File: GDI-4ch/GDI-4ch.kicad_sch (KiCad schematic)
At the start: 311 parts, among them J1 Conn_02x02_Odd_Even, J2 FTSH-107-01-F-DV-K, J3 TC2030, J4 Conn_01x06, J5 Conn_01x06, P1 368255-2, P18 Pad, P19 Pad, P2 Pad, P20 Pad, P3 Pad, P36 Pad, P4 Pad, P5 Pad, Q1 BUK9230-100B, Q10 BUK9230-100B, Q11 BUK9230-100B, Q12 BUK9230-100B, Q13 AOD4185, Q14 VND14NV04TR-E, Q15 VND14NV04TR-E, Q16 BUK9230-100B, Q2 BUK9230-100B, Q3 BUK9230-100B, Q4 BUK9230-100B, Q5 BUK9230-100B, Q6 BUK9230-100B, Q7 BUK9230-100B, Q8 BUK9230-100B, Q9 BUK9230-100B, U1 MC33816, U2 TJA1051T-3, U3 LM78M05_TO252, U4 74HC14PW,118, U5 XC6206P332MR, U6 MCP6004, U7 GD32F103CBT6, U8 74HC14PW,118, Y1 8MHz, Y2 1MHz

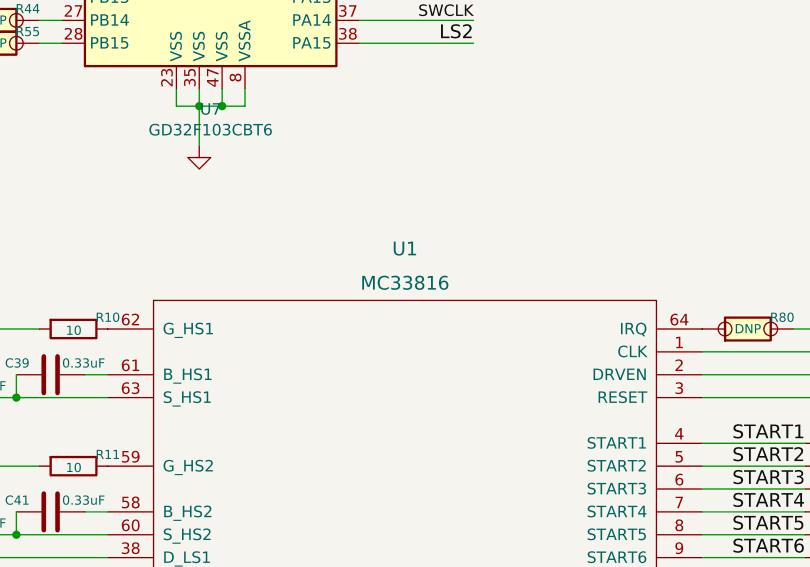
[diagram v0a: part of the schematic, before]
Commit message: #205
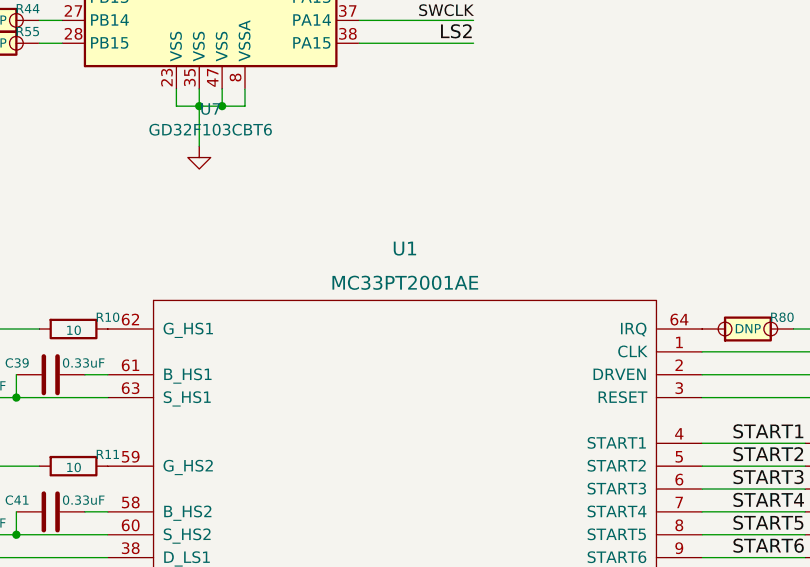
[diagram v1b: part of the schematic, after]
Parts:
- P1: LCSC (none) -> C392284
- U1: value MC33816 -> MC33PT2001AE; LCSC (none) -> C729087
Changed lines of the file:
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@@
       (effects (font (size 1.27 1.27)) hide)
     )
+    (property "LCSC" "C392284" (at 25.4 212.09 0)
+      (effects (font (size 1.524 1.524)) hide)
+    )
     (pin "1")
     (pin "114")
@@
       (effects (font (size 1.27 1.27)) hide)
     )
+    (property "LCSC" "C392284" (at 26.67 29.21 0)
+      (effects (font (size 1.524 1.524)) hide)
+    )
     (pin "1")
     (pin "114")
@@
       (effects (font (size 1.524 1.524)))
     )
-    (property "Value" "MC33816" (at 403.86 135.89 0)
+    (property "Value" "MC33PT2001AE" (at 403.86 135.89 0)
       (effects (font (size 1.524 1.524)))
     )
@@
       (effects (font (size 1.524 1.524)) hide)
     )
+    (property "LCSC" "C729087" (at 403.86 212.09 0)
+      (effects (font (size 1.524 1.524)) hide)
+    )

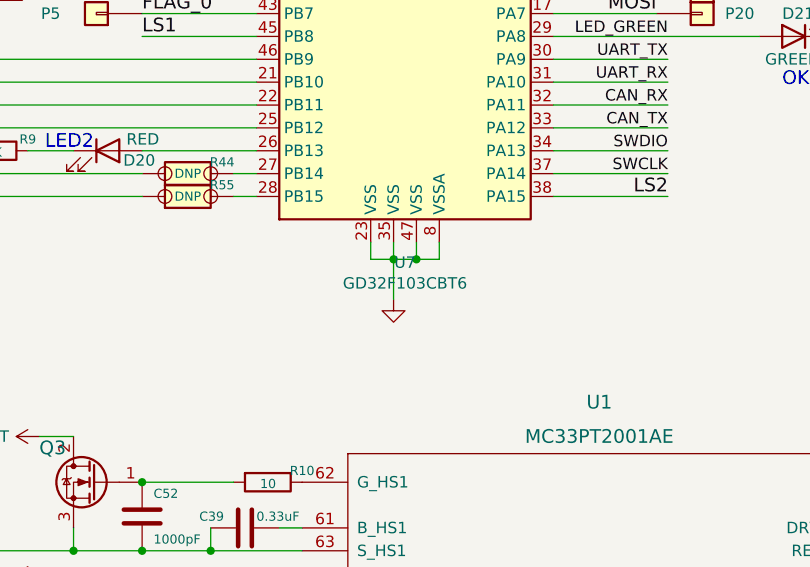
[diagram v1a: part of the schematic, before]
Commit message: #224, #225 re-fab
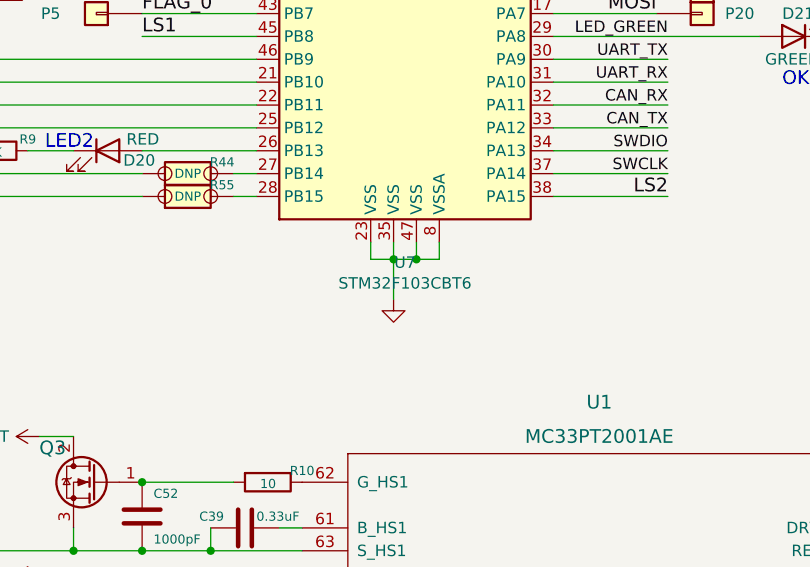
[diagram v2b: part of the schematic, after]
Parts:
- J4, J5: LCSC C5156615 -> C37208
- S7, S8: LCSC C115357 -> C455280
- U7: value GD32F103CBT6 -> STM32F103CBT6; LCSC C77979 -> C8304
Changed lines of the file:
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@@
       (effects (font (size 1.27 1.27)) hide)
     )
-    (property "LCSC" "C5156615" (at 551.18 121.92 0)
+    (property "LCSC" "C37208" (at 551.18 121.92 0)
       (effects (font (size 1.524 1.524)) hide)
     )
@@
       (effects (font (size 1.27 1.27)) hide)
     )
-    (property "LCSC" "C115357" (at 340.995 16.51 0)
+    (property "LCSC" "C455280" (at 340.995 16.51 0)
       (effects (font (size 1.27 1.27)) hide)
     )
@@
       (effects (font (size 1.27 1.27)) hide)
     )
-    (property "LCSC" "C115357" (at 341.63 35.56 0)
+    (property "LCSC" "C455280" (at 341.63 35.56 0)
       (effects (font (size 1.27 1.27)) hide)
     )
@@
       (effects (font (size 1.27 1.27)) hide)
     )
-    (property "LCSC" "C5156615" (at 107.95 46.99 0)
+    (property "LCSC" "C37208" (at 107.95 46.99 0)
       (effects (font (size 1.524 1.524)) hide)
     )
@@
       (effects (font (size 1.27 1.27)))
     )
-    (property "Value" "GD32F103CBT6" (at 382.27 118.872 0)
+    (property "Value" "STM32F103CBT6" (at 382.27 118.872 0)
       (effects (font (size 1.27 1.27)))
     )
@@
       (effects (font (size 1.27 1.27)) hide)
     )
-    (property "LCSC" "C77979" (at 383.54 76.2 0)
+    (property "LCSC" "C8304" (at 383.54 76.2 0)
       (effects (font (size 1.524 1.524)) hide)
     )
